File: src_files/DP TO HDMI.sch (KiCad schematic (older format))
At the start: 38 parts, among them J8 2001-1-2-21-00-BK, U12 MCDP2900, U13 ZLDO1117G12TA, U14 ESD5304D-TP, U15 ESD5304D-TP, U16 ESD5304D-TP, Y4 27MHz

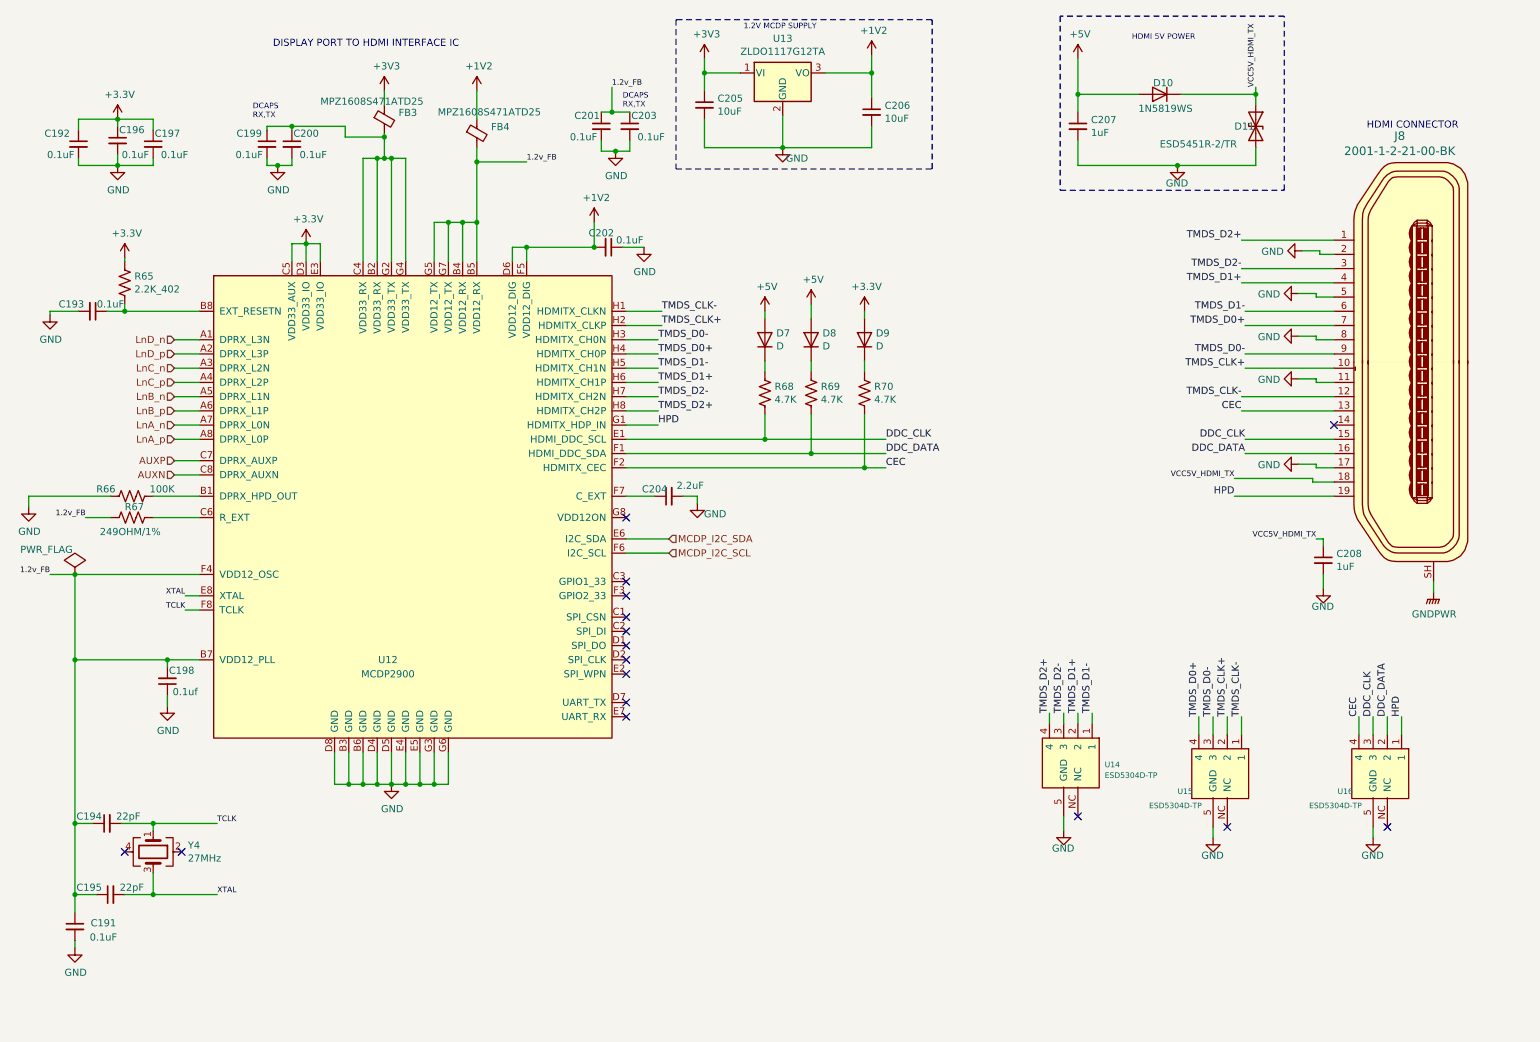
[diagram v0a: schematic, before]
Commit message: updated footprint and schematics
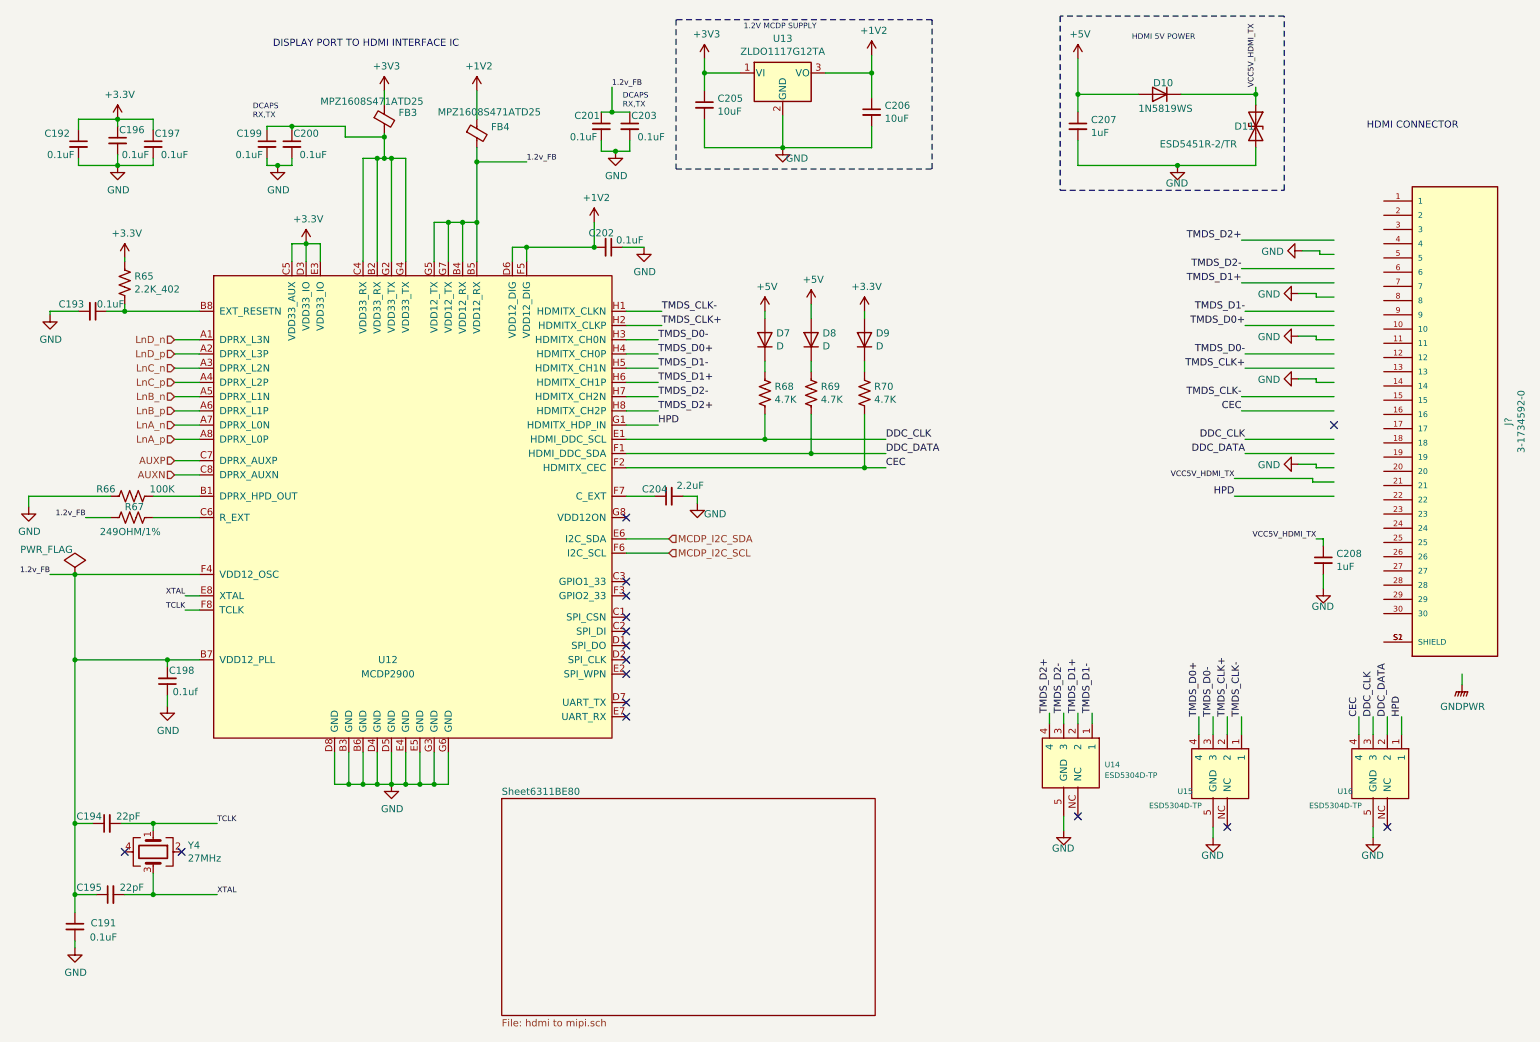
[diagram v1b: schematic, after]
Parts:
- removed J8: 2001-1-2-21-00-BK, digikey-footprints:HDMI_Mini_Female_2001-1-2-21-00-BK, symbol dk_USB-DVI-HDMI-Connectors:2001-1-2-21-00-BK
- added J?: 3-1734592-0, greencharge-footprints:TE_3-1734592-0, symbol 3-1734592-0:3-1734592-0
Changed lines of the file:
@@
 $Descr A4 11693 8268
 encoding utf-8
-Sheet 7 15
+Sheet 7 16
 Title ""
 Date ""
@@
 NoConn ~ 9100 6200
 $Comp
-L dk_USB-DVI-HDMI-Connectors:2001-1-2-21-00-BK J?
-U 1 1 637EF133
-P 10450 2975
-AR Path="/61C73AB6/637EF133" Ref="J?"  Part="1"
-AR Path="/61C73AB6/635B9242/637EF133" Ref="J8"  Part="1"
-F 0 "J8" H 10588 4607 60  0000 C CNN
-F 1 "2001-1-2-21-00-BK" H 10588 4501 60  0000 C CNN
-F 2 "digikey-footprints:HDMI_Mini_Female_2001-1-2-21-00-BK" H 10650 3175 60  0001 L CNN
-F 3 "http://cnctech.us/pdfs/2001-1-2-21-00-BK.pdf" H 10650 3275 60  0001 L CNN
-F 4 "1175-1704-1-ND" H 10650 3375 60  0001 L CNN "Digi-Key_PN"
-F 5 "2001-1-2-21-00-BK" H 10650 3475 60  0001 L CNN "MPN"
-F 6 "Connectors, Interconnects" H 10650 3575 60  0001 L CNN "Category"
-F 7 "USB, DVI, HDMI Connectors" H 10650 3675 60  0001 L CNN "Family"
-F 8 "http://cnctech.us/pdfs/2001-1-2-21-00-BK.pdf" H 10650 3775 60  0001 L CNN "DK_Datasheet_Link"
-F 9 "/product-detail/en/cnc-tech/2001-1-2-21-00-BK/1175-1704-1-ND/4867013" H 10650 3875 60  0001 L CNN "DK_Detail_Page"
-F 10 "CONN RCPT MINI HDMI 19POS SMD RA" H 10650 3975 60  0001 L CNN "Description"
-F 11 "CNC Tech" H 10650 4075 60  0001 L CNN "Manufacturer"
-F 12 "Active" H 10650 4175 60  0001 L CNN "Status"
-	1    10450 2975
-	-1   0    0    -1
-$EndComp
-$Comp
 L OLIMEX_Power:GND #PWR?
 U 1 1 637EF13C
@@
 Wire Wire Line
 	9850 2075 9200 2075
-$Comp
-L power:GNDPWR #PWR?
-U 1 1 637EF181
-P 10550 4550
-AR Path="/61C73AB6/637EF181" Ref="#PWR?"  Part="1"
-AR Path="/61C73AB6/635B9242/637EF181" Ref="#PWR0207"  Part="1"
-F 0 "#PWR0207" H 10550 4350 50  0001 C CNN
-F 1 "GNDPWR" H 10554 4396 50  0000 C CNN
-F 2 "" H 10550 4500 50  0001 C CNN
-F 3 "" H 10550 4500 50  0001 C CNN
-	1    10550 4550
-	1    0    0    -1
-$EndComp
-Wire Wire Line
-	10550 4550 10550 4475
 $Comp
 L Device:C_Small C?
@@
 	0    -1   -1   0
 $EndComp
+Wire Wire Line
+	10750 5200 10750 5125
+$Comp
+L power:GNDPWR #PWR?
+U 1 1 637EF181
+P 10750 5200
+AR Path="/61C73AB6/637EF181" Ref="#PWR?"  Part="1"
+AR Path="/61C73AB6/635B9242/637EF181" Ref="#PWR0207"  Part="1"
+F 0 "#PWR0207" H 10750 5000 50  0001 C CNN
+F 1 "GNDPWR" H 10754 5046 50  0000 C CNN
+F 2 "" H 10750 5150 50  0001 C CNN
+F 3 "" H 10750 5150 50  0001 C CNN
+	1    10750 5200
+	1    0    0    -1
+$EndComp
+$Sheet
+S 4000 6000 2625 1525
+U 6311BE81
+F0 "Sheet6311BE80" 50
+F1 "hdmi to mipi.sch" 50
+$EndSheet
+$Comp
+L 3-1734592-0:3-1734592-0 J?
+U 1 1 631A8114
+P 10700 3300
+AR Path="/631A8114" Ref="J?"  Part="1"
+AR Path="/61C73AB6/631A8114" Ref="J?"  Part="1"
+AR Path="/62F6D336/631A8114" Ref="J?"  Part="1"
+AR Path="/61C73AB6/635B9242/631A8114" Ref="J?"  Part="1"
+F 0 "J?" V 11075 3250 50  0000 C CNN
+F 1 "3-1734592-0" V 11166 3250 50  0000 C CNN
+F 2 "greencharge-footprints:TE_3-1734592-0" H 10700 3300 50  0001 L BNN
+F 3 "" H 10700 3300 50  0001 L BNN
+F 4 "TE Connectivity" H 10700 3300 50  0001 L BNN "MANUFACTURER"
+F 5 "2.05mm" H 10700 3300 50  0001 L BNN "MAXIMUM_PACKAGE_HEIGHT"
+F 6 "Manufacturer Recommendations" H 10700 3300 50  0001 L BNN "STANDARD"
+F 7 "C" H 10700 3300 50  0001 L BNN "PARTREV"
+	1    10700 3300
+	1    0    0    -1
+$EndComp
 $EndSCHEMATC
